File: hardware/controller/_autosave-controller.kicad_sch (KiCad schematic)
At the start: 41 parts, among them J1 USB_C_Receptacle_PowerOnly_6P, J2 Bat, J3 Conn_01x06, Q1 AO3401, Q2 AllPower__AP2300, Q3 AllPower__AP2300, SW1 TS-1199A-B-B, SW2 RKJXV1224005, SW3 RKJXV1224005, SW4 SW_Push, SW5 TS-1199A-B-B, SW6 SW_Push, U1 TP4059, U3 XC6220B331MR, U4 ESP32-C3-WROOM-02-N4

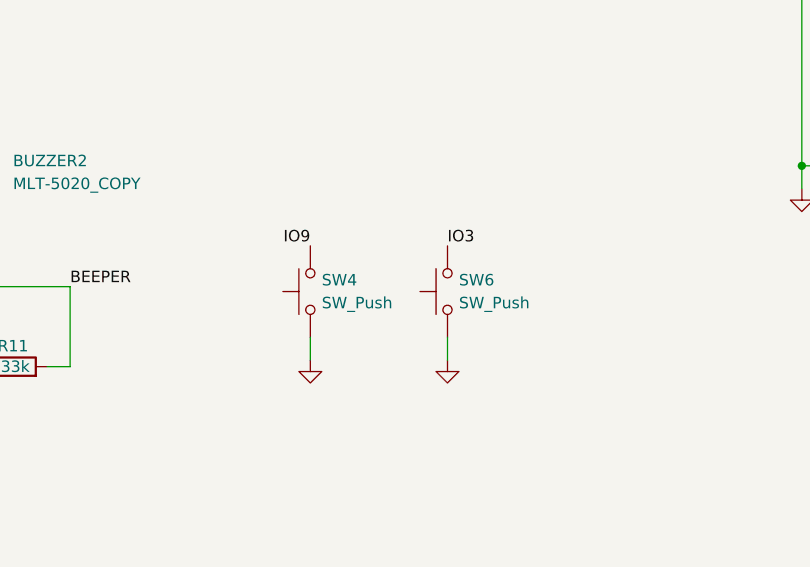
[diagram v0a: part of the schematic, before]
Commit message: update controller
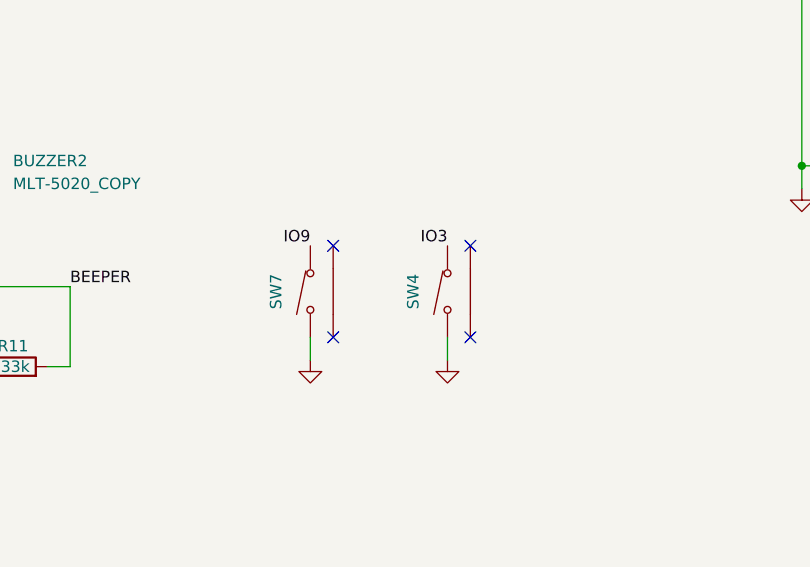
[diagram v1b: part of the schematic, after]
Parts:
- removed SW4, SW6: SW_Push, symbol Switch:SW_Push
- added SW4, SW7: TC-1102N-C-AS-B, espController:SW-TH_TC-1102N-C-AS-B, symbol espController:TC-1102N-C-AS-B
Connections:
- net GND: now also SW4.1, SW7.1
- net IO3: now also SW4.2
- net IO9: now also SW7.2
- no-connect marks 3 -> 7
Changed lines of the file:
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@@
 		(at 52.07 49.53)
 	)
+	(no_connect
+		(at 120.65 88.9)
+	)
+	(no_connect
+		(at 135.89 99.06)
+	)
+	(no_connect
+		(at 120.65 99.06)
+	)
+	(no_connect
+		(at 135.89 88.9)
+	)
 	(wire
 		(pts
@@
 	)
 	(label "IO3"
-		(at 133.35 88.9 0)
+		(at 133.35 88.9 180)
 		(fields_autoplaced yes)
 		(effects
@@
 				(size 1.27 1.27)
 			)
-			(justify left bottom)
+			(justify right bottom)
 		)
 	)
@@
 	)
 	(symbol
-		(lib_id "Switch:SW_Push")
-		(at 118.11 93.98 90)
-		(unit 1)
-		(exclude_from_sim no)
-		(in_bom yes)
-		(on_board yes)
-		(dnp no)
-		(fields_autoplaced yes)
-		(property "Reference" "SW4"
-			(at 119.38 92.7099 90)
-			(effects
-				(font
-					(size 1.27 1.27)
-				)
-				(justify right)
-			)
-		)
-		(property "Value" "SW_Push"
-			(at 119.38 95.2499 90)
-			(effects
-				(font
-					(size 1.27 1.27)
-				)
-				(justify right)
-			)
-		)
-		(property "Footprint" ""
-			(at 113.03 93.98 0)
-			(effects
-				(font
-					(size 1.27 1.27)
-				)
-				(hide yes)
-			)
-		)
-		(property "Datasheet" "~"
-			(at 113.03 93.98 0)
-			(effects
-				(font
-					(size 1.27 1.27)
-				)
-				(hide yes)
-			)
-		)
-		(property "Description" "Push button switch, generic, two pins"
-			(at 118.11 93.98 0)
-			(effects
-				(font
-					(size 1.27 1.27)
-				)
-				(hide yes)
-			)
-		)
-		(pin "1"
-		)
-		(pin "2"
-		)
-		(instances
-			(project "controller"
-				(path "/ac6122ee-da02-46ca-bfd7-d634b1b1f53e"
-					(reference "SW4")
-					(unit 1)
-				)
-			)
-		)
-	)
-	(symbol
 		(lib_id "Mechanical:MountingHole")
 		(at 40.64 132.08 0)
@@
 	)
 	(symbol
+		(lib_id "espController:TC-1102N-C-AS-B")
+		(at 133.35 93.98 90)
+		(unit 1)
+		(exclude_from_sim no)
+		(in_bom yes)
+		(on_board yes)
+		(dnp no)
+		(property "Reference" "SW4"
+			(at 129.54 93.98 0)
+			(effects
+				(font
+					(size 1.27 1.27)
+				)
+			)
+		)
+		(property "Value" "TC-1102N-C-AS-B"
+			(at 129.54 93.98 0)
+			(effects
+				(font
+					(size 1.27 1.27)
+				)
+				(hide yes)
+			)
+		)
+		(property "Footprint" "espController:SW-TH_TC-1102N-C-AS-B"
+			(at 134.366 93.98 0)
+			(effects
+				(font
+					(size 1.27 1.27)
+				)
+				(hide yes)
+			)
+		)
+		(property "Datasheet" "http://www.szlcsc.com/product/details_393914.html"
+			(at 139.446 93.98 0)
+			(effects
+				(font
+					(size 1.27 1.27)
+				)
+				(hide yes)
+			)
+		)
+		(property "Description" "C406151"
+			(at 144.526 93.98 0)
+			(effects
+				(font
+					(size 1.27 1.27)
+				)
+				(hide yes)
+			)
+		)
+		(property "uuid" "std:62ddec029f9448109c55e50d5022673b"
+			(at 144.526 93.98 0)
+			(effects
+				(font
+					(size 1.27 1.27)
+				)
+				(hide yes)
+			)
+		)
+		(pin "4"
+		)
+		(pin "3"
+		)
+		(pin "2"
+		)
+		(pin "1"
+		)
+		(instances
+			(project "controller"
+				(path "/ac6122ee-da02-46ca-bfd7-d634b1b1f53e"
+					(reference "SW4")
+					(unit 1)
+				)
+			)
+		)
+	)
+	(symbol
 		(lib_id "Device:LED")
 		(at 213.36 38.1 90)
@@
 	)
 	(symbol
+		(lib_id "espController:TC-1102N-C-AS-B")
+		(at 118.11 93.98 90)
+		(unit 1)
+		(exclude_from_sim no)
+		(in_bom yes)
+		(on_board yes)
+		(dnp no)
+		(property "Reference" "SW7"
+			(at 114.3 93.98 0)
+			(effects
+				(font
+					(size 1.27 1.27)
+				)
+			)
+		)
+		(property "Value" "TC-1102N-C-AS-B"
+			(at 114.3 93.98 0)
+			(effects
+				(font
+					(size 1.27 1.27)
+				)
+				(hide yes)
+			)
+		)
+		(property "Footprint" "espController:SW-TH_TC-1102N-C-AS-B"
+			(at 119.126 93.98 0)
+			(effects
+				(font
+					(size 1.27 1.27)
+				)
+				(hide yes)
+			)
+		)
+		(property "Datasheet" "http://www.szlcsc.com/product/details_393914.html"
+			(at 124.206 93.98 0)
+			(effects
+				(font
+					(size 1.27 1.27)
+				)
+				(hide yes)
+			)
+		)
+		(property "Description" "C406151"
+			(at 129.286 93.98 0)
+			(effects
+				(font
+					(size 1.27 1.27)
+				)
+				(hide yes)
+			)
+		)
+		(property "uuid" "std:62ddec029f9448109c55e50d5022673b"
+			(at 129.286 93.98 0)
+			(effects
+				(font
+					(size 1.27 1.27)
+				)
+				(hide yes)
+			)
+		)
+		(pin "4"
+		)
+		(pin "3"
+		)
+		(pin "2"
+		)
+		(pin "1"
+		)
+		(instances
+			(project "controller"
+				(path "/ac6122ee-da02-46ca-bfd7-d634b1b1f53e"
+					(reference "SW7")
+					(unit 1)
+				)
+			)
+		)
+	)
+	(symbol
 		(lib_id "power:GND")
 		(at 217.17 113.03 180)
@@
 					(unit 1)
 				)
-			)
-		)
-	)
-	(symbol
-		(lib_id "Switch:SW_Push")
-		(at 133.35 93.98 90)
-		(unit 1)
-		(exclude_from_sim no)
-		(in_bom yes)
-		(on_board yes)
-		(dnp no)
-		(fields_autoplaced yes)
-		(property "Reference" "SW6"
-			(at 134.62 92.7099 90)
-			(effects
-				(font
-					(size 1.27 1.27)
-				)
-				(justify right)
-			)
-		)
-		(property "Value" "SW_Push"
-			(at 134.62 95.2499 90)
-			(effects
-				(font
-					(size 1.27 1.27)
-				)
-				(justify right)
-			)
-		)
-		(property "Footprint" ""
-			(at 128.27 93.98 0)
-			(effects
-				(font
-					(size 1.27 1.27)
-				)
-				(hide yes)
-			)
-		)
-		(property "Datasheet" "~"
-			(at 128.27 93.98 0)
-			(effects
-				(font
-					(size 1.27 1.27)
-				)
-				(hide yes)
-			)
-		)
-		(property "Description" "Push button switch, generic, two pins"
-			(at 133.35 93.98 0)
-			(effects
-				(font
-					(size 1.27 1.27)
-				)
-				(hide yes)
-			)
-		)
-		(pin "1"
-		)
-		(pin "2"
-		)
-		(instances
-			(project "controller"
-				(path "/ac6122ee-da02-46ca-bfd7-d634b1b1f53e"
-					(reference "SW6")
-					(unit 1)
-				)
